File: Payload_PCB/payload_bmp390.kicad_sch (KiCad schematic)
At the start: 5 parts, among them IC1 BMP390

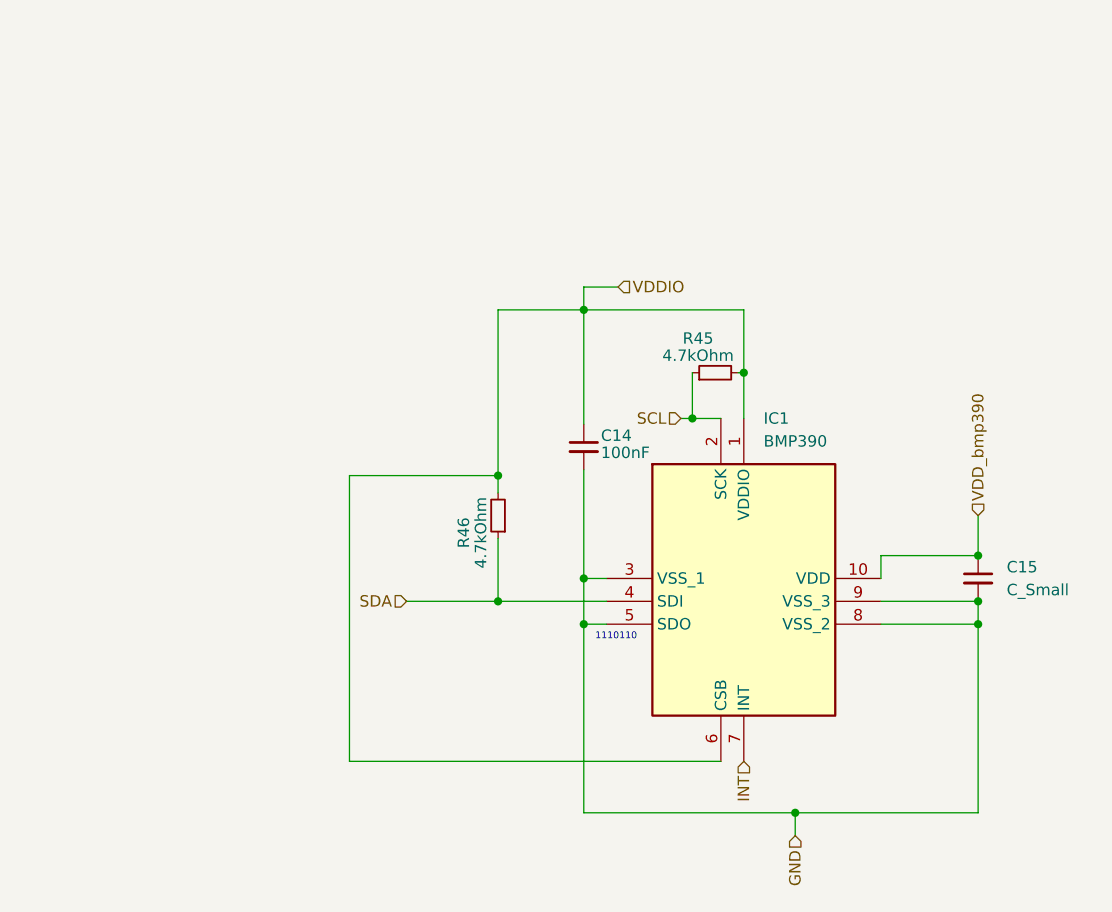
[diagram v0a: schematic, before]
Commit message: Adjust page size
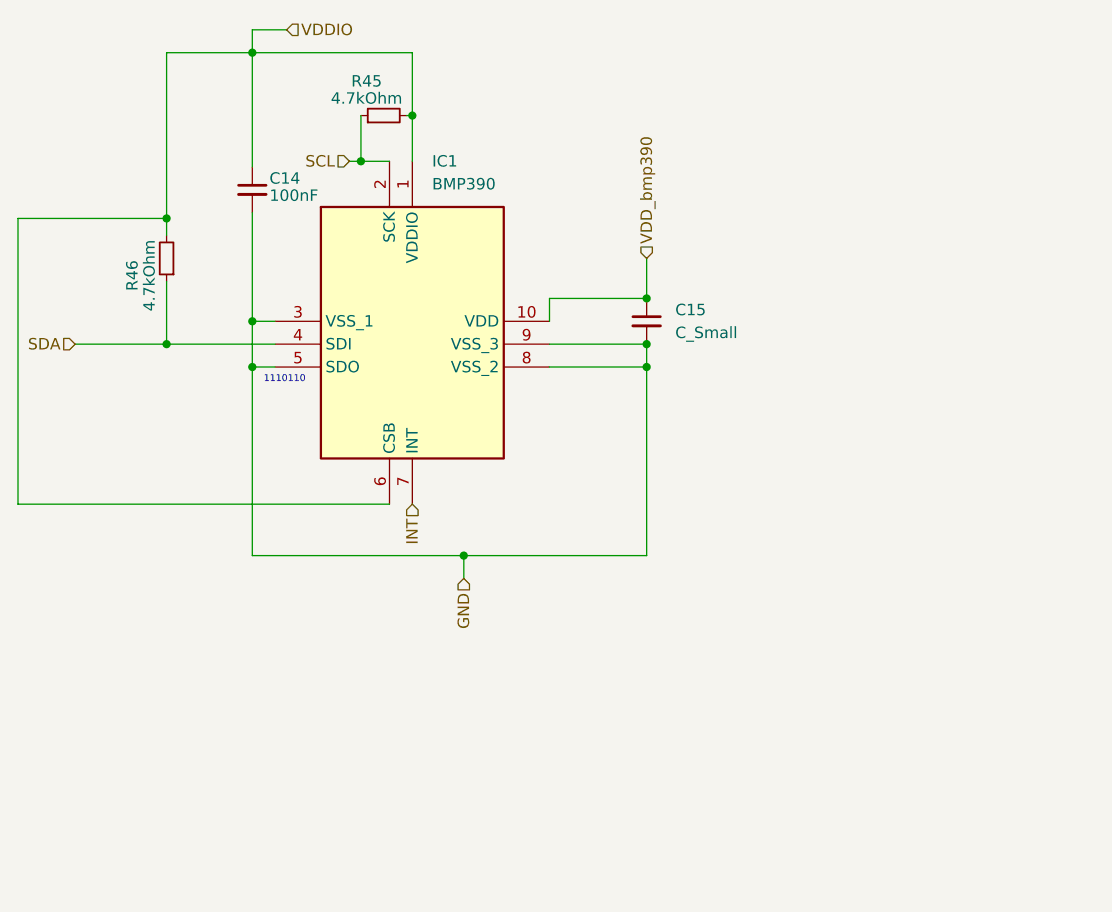
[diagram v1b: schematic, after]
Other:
- moved on the sheet: C14, C15, IC1, R45, R46
